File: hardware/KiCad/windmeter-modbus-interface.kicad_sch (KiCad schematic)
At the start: 22 parts, among them J1 MODBUS-P1, J2 Programming, J3 MODBUS-P2, U1 CH32V003J4M6, U2 MAX3485

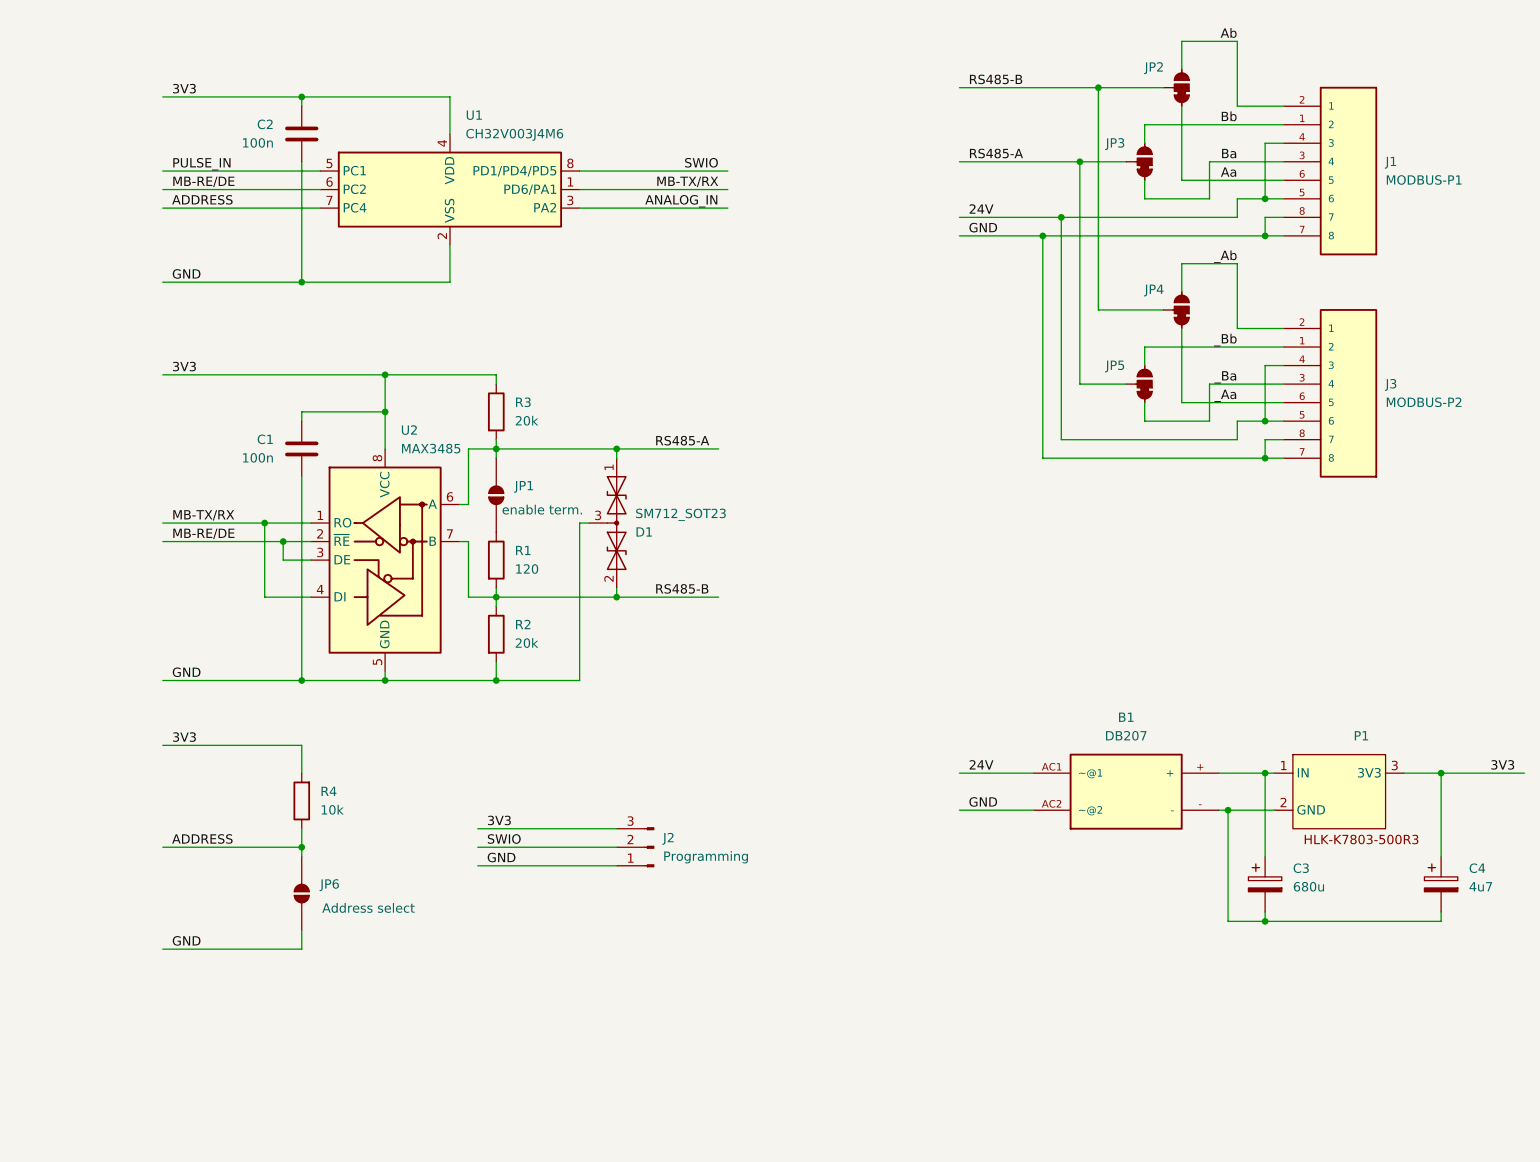
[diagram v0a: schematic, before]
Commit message: First scaffolding
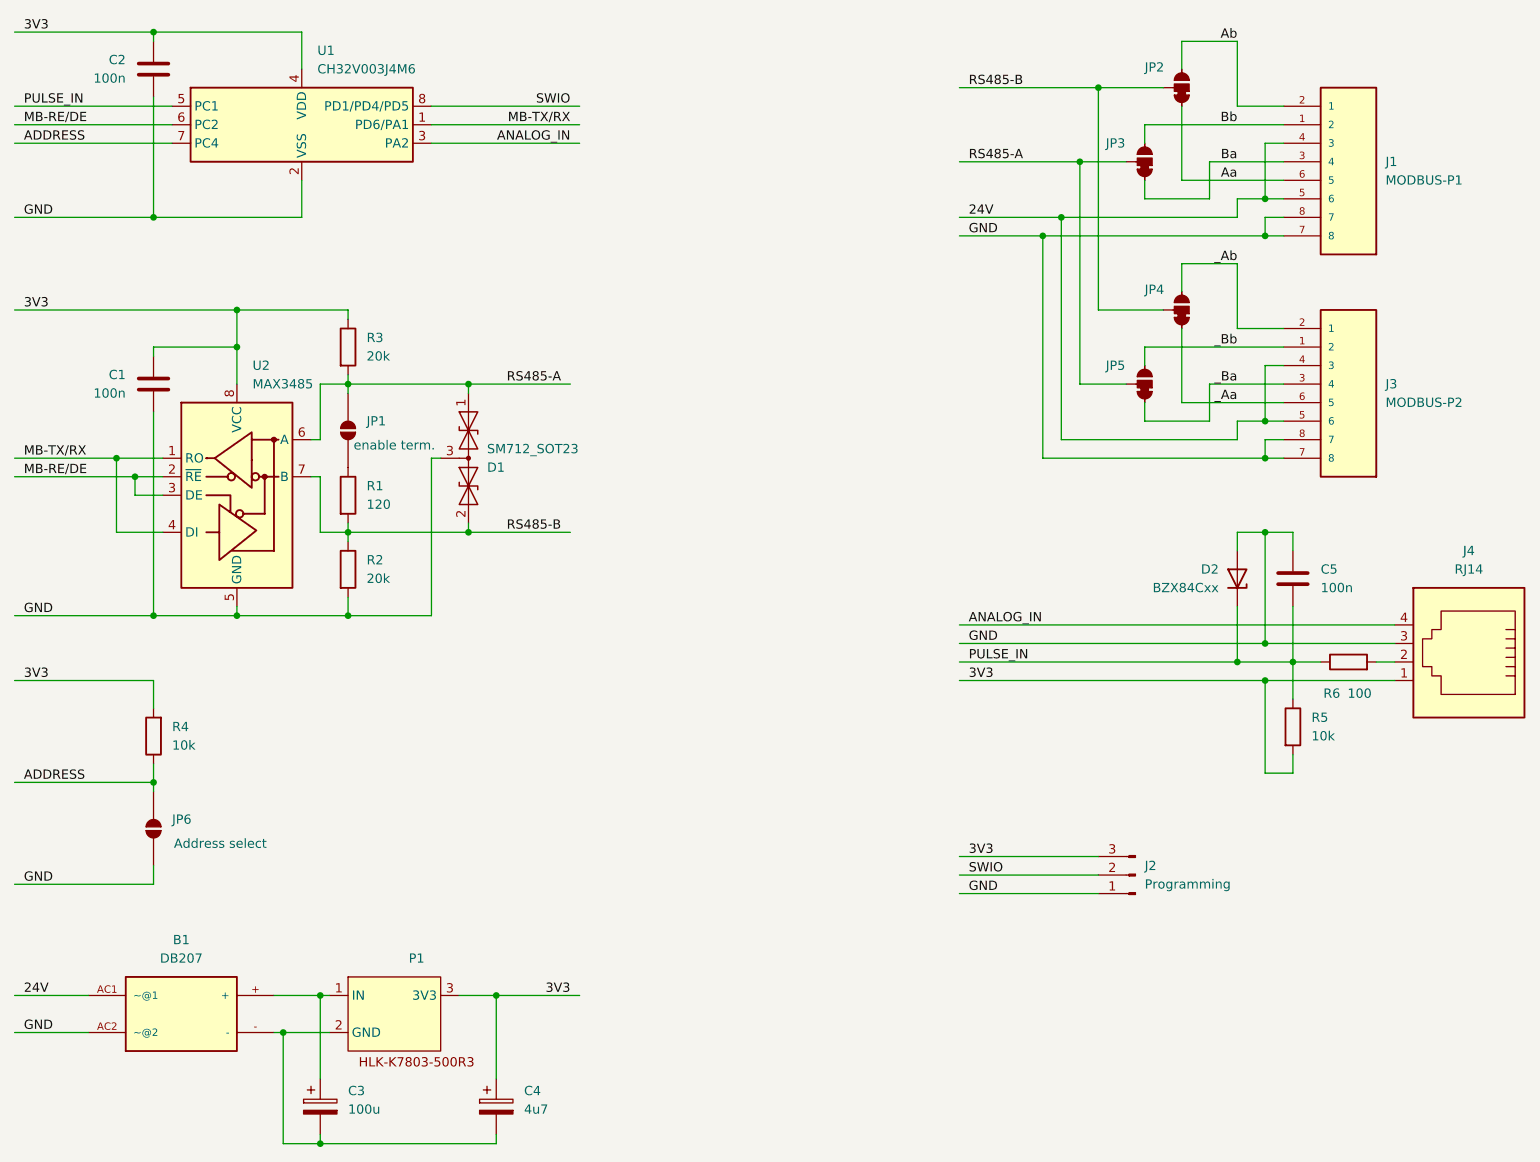
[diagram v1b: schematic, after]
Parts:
- added C5: 100n, Capacitor_SMD:C_1206_3216Metric_Pad1.33x1.80mm_HandSolder, symbol Device:C
- added D2: BZX84Cxx, Package_TO_SOT_SMD:SOT-23, symbol Diode:BZX84Cxx
- added J4: RJ14, symbol Connector:RJ14
- added R5: 10k, Resistor_SMD:R_1206_3216Metric_Pad1.30x1.75mm_HandSolder, symbol Device:R
- added R6: 100, Resistor_SMD:R_1206_3216Metric_Pad1.30x1.75mm_HandSolder, symbol Device:R
- C3: value 680u -> 100u
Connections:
- net 3V3: now also J4.1, R5.2
- net ANALOG_IN: now also J4.4
- net GND: now also C5.1, D2.1 (A), J4.3
- net PULSE_IN: now also C5.2, D2.3 (K), R5.1, R6.1
- new net: J4.2, R6.2
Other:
- company: (none) -> RFSee
- title: (none) -> Windmeter interface for Modbus RS458
- moved on the sheet: B1, C1, C2, C3, C4, D1, J2, JP1, JP6, P1, R1, R2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
